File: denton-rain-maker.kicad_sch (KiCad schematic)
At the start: 73 parts, among them J1 Live(AC2), J2 Neutral(AC1), J3 SEED C3, Q1 BT136S-800E, Q2 BT136S-800E, Q3 BT136S-800E, Q4 BT136S-800E, SW1 SW_Rotary_1x8_MP, U1 MOC3063M, U2 MOC3063M, U3 MOC3063M, U4 MOC3063M, U5 LM5164DDA

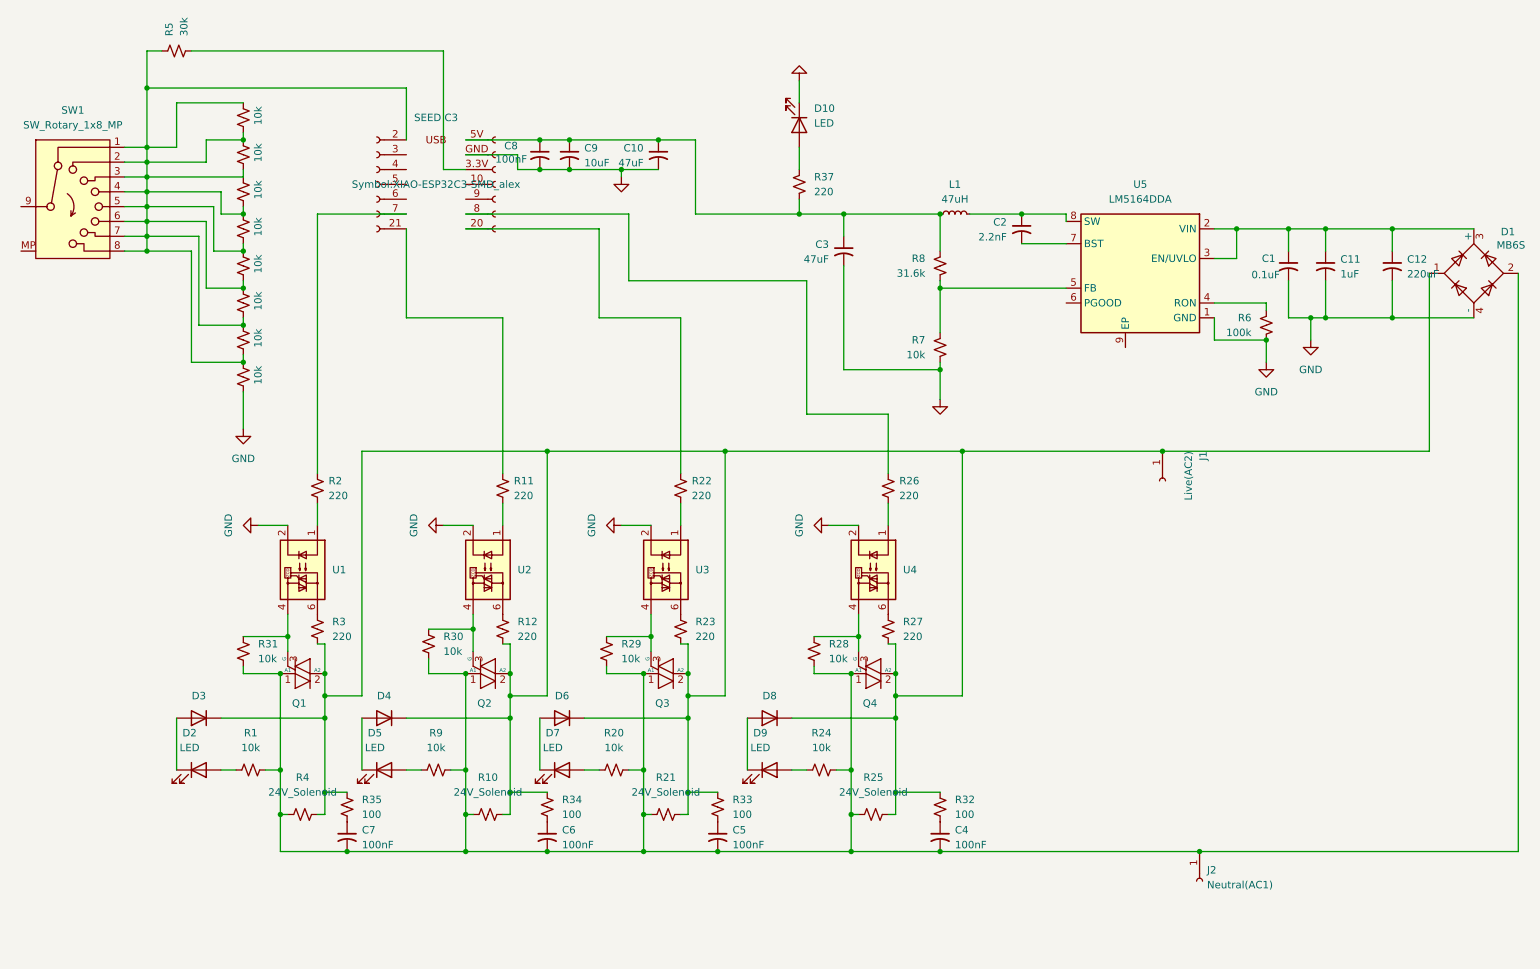
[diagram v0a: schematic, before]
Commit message: starting on layout
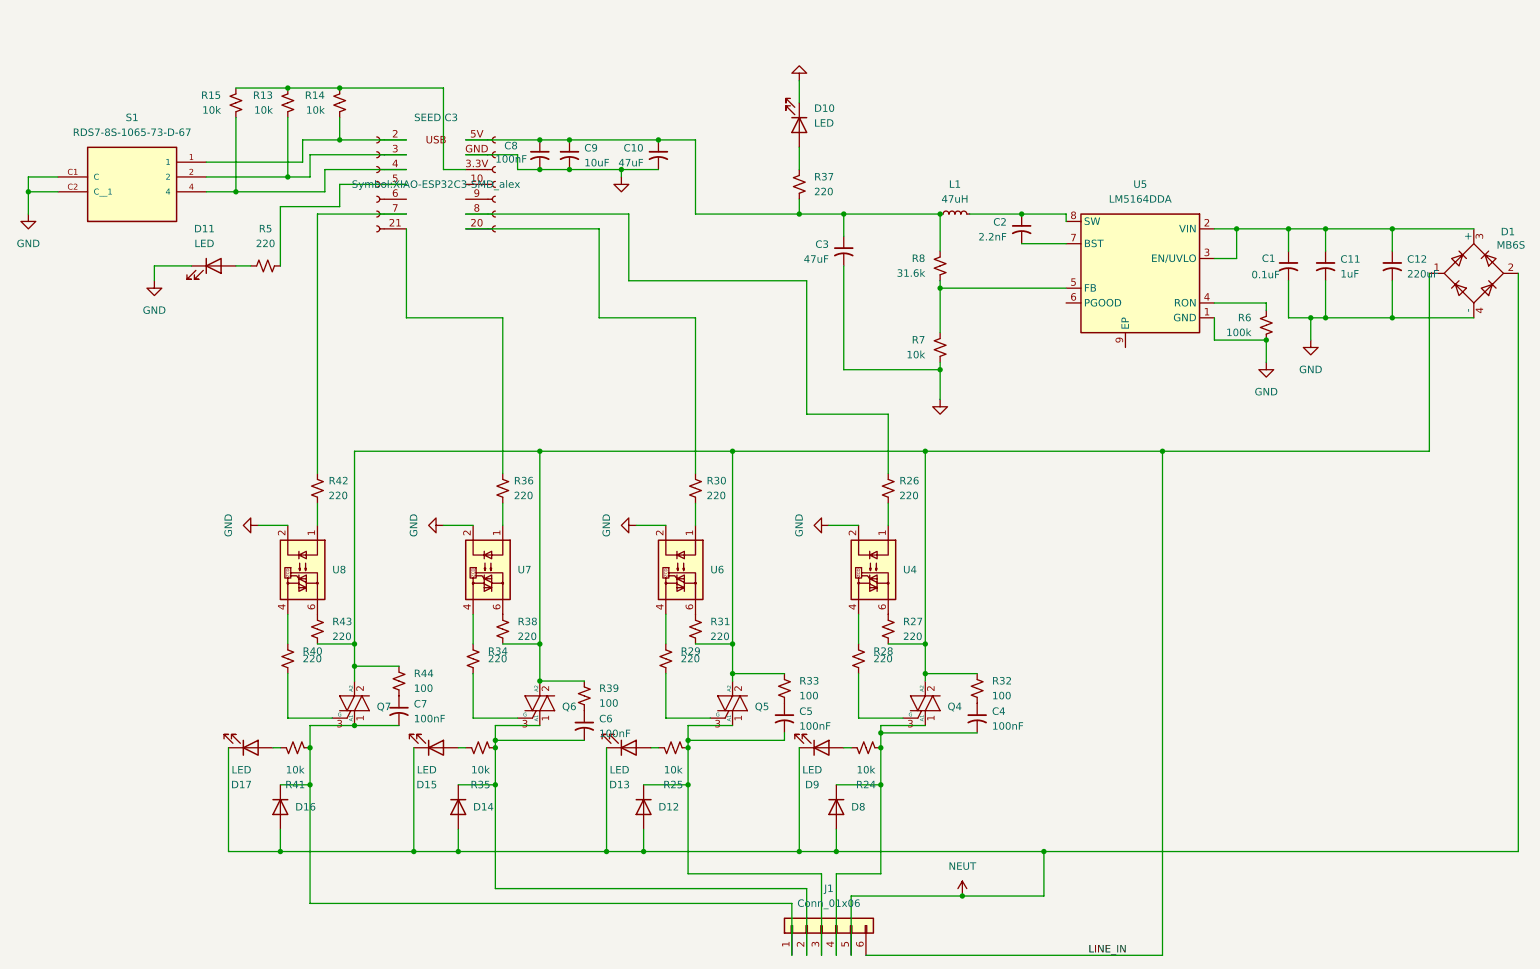
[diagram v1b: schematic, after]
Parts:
- removed D2, D5, D7: LED, LED_SMD:LED_1206_3216Metric_Pad1.42x1.75mm_HandSolder, symbol Device:LED
- removed D3, D4, D6: 1N4148W, Diode_SMD:D_SOD-123, symbol Diode:1N4148W
- removed J1: Live(AC2), Connector_PinSocket_1.27mm:PinSocket_1x01_P1.27mm_Vertical, symbol Connector:Conn_01x01_Socket
- removed J2: Neutral(AC1), Connector_PinSocket_1.27mm:PinSocket_1x01_P1.27mm_Vertical, symbol Connector:Conn_01x01_Socket
- removed Q1, Q2, Q3: BT136S-800E, Package_TO_SOT_SMD:TO-252-3_TabPin2, symbol Triac_Thyristor:BT136-800
- removed R1, R16, R17, R18, R19, R20, R9: 10k, Resistor_SMD:R_1206_3216Metric_Pad1.30x1.75mm_HandSolder, symbol Device:R_Small_US
- removed R10, R21, R4: 24V_Solenoid, symbol Device:R_Small_US
- removed R11, R12, R2, R22, R23, R3: 220, Resistor_SMD:R_1206_3216Metric_Pad1.30x1.75mm_HandSolder, symbol Device:R_Small_US
- removed SW1: SW_Rotary_1x8_MP, symbol Switch:SW_Rotary_1x8_MP
- removed U1, U2, U3: MOC3063M, Package_DIP:DIP-6_W7.62mm, symbol Relay_SolidState:MOC3063M
- added D11, D13, D15, D17: LED, LED_THT:LED_D3.0mm, symbol Device:LED
- added D12, D14, D16: 1N4148W, Diode_SMD:D_SOD-123, symbol Diode:1N4148W
- added J1: Conn_01x06, TerminalBlock_Phoenix:TerminalBlock_Phoenix_MPT-0,5-6-2.54_1x06_P2.54mm_Horizontal, symbol Connector_Generic:Conn_01x06
- added Q5, Q6, Q7: BT136S-800E, Package_TO_SOT_SMD:TO-252-3_TabPin2, symbol Triac_Thyristor:BT136-800
- added R38, R40, R42, R43: 220, Resistor_SMD:R_1206_3216Metric_Pad1.30x1.75mm_HandSolder, symbol Device:R_Small_US
- added R39, R44: 100, Resistor_SMD:R_1206_3216Metric_Pad1.30x1.75mm_HandSolder, symbol Device:R_Small_US
- added R41: 10k, Resistor_SMD:R_1206_3216Metric_Pad1.30x1.75mm_HandSolder, symbol Device:R_Small_US
- added S1: RDS7-8S-1065-73-D-67, Downloads:SW_RDS7-8S-1065-73-D-67, symbol RDS7-8S-1065-73-D-67:RDS7-8S-1065-73-D-67
- added U6, U7, U8: MOC3063M, Package_DIP:DIP-6_W7.62mm, symbol Relay_SolidState:MOC3063M
- D10: footprint (none) -> LED_THT:LED_D3.0mm
- D9: footprint LED_SMD:LED_1206_3216Metric_Pad1.42x1.75mm_HandSolder -> LED_THT:LED_D3.0mm
- R25: value 24V_Solenoid -> 10k; footprint (none) -> Resistor_SMD:R_1206_3216Metric_Pad1.30x1.75mm_HandSolder
- R28, R29, R30, R31, R36: value 10k -> 220
- R34: value 100 -> 220
- R35: value 100 -> 10k
- R5: value 30k -> 220
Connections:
- net GND: now also D11.1 (K), S1.C1 (C), S1.C2 (C__1), U6.2, U7.2, U8.2; no longer R36.1
- net at J3.20 (Pin_7): now also R30.2
- net at R31.1: now also U6.6
- net LINE_IN: now reaches D1.1, Q4.2 (A2), R27.2, R32.1, R33.1
- net LINE_IN: now also R31.2, J1.6 (Pin_6), Q5.2 (A2), Q6.2 (A2), Q7.2 (A2), R38.2, R39.1, R43.2, R44.1; no longer D8.1 (K), R25.1, R34.1, R35.1
- net at J3.7 (Pin_3): now also R42.2
- net at R28.1, U4.4: no longer Q4.3 (G)
- net NEUT: now reaches D8.2 (A), D9.1 (K)
- net NEUT: now also D1.2, D12.2 (A), D13.1 (K), D14.2 (A), D15.1 (K), D16.2 (A), D17.1 (K), J1.5 (Pin_5)
- net at R30.1: now also U6.1
- net at C6.1: now also R39.2; no longer R34.2
- net at R35.2: now also C6.2, D14.1 (K), J1.2 (Pin_2), Q6.1 (A1); no longer C7.1
- net at R29.1: now also U6.4
- net at J3.3.3V (Pin_3): now also R13.1, R14.1, R15.1; no longer R5.1
- net at J3.21 (Pin_2): now also R36.2
- net at J3.3 (Pin_7): now also R13.2, S1.2
- net at J3.4 (Pin_6): now also R15.2, S1.4
- net at J3.5 (Pin_5): now also R5.2
- new net: J3.2 (Pin_8), R14.2, S1.1
- new net: C7.1, R44.2
- new net: C7.2, D16.1 (K), J1.1 (Pin_1), Q7.1 (A1), R41.2
- new net: C5.2, D12.1 (K), J1.3 (Pin_3), Q5.1 (A1), R25.2
- new net: Q5.3 (G), R29.2
- new net: C4.2, D8.1 (K), J1.4 (Pin_4), Q4.1 (A1), R24.2
- new net: Q4.3 (G), R28.2
- new net: D17.2 (A), R41.1
- new net: R36.1, U7.1
- new net: R34.1, U7.4
- new net: R38.1, U7.6
- new net: Q6.3 (G), R34.2
- new net: D13.2 (A), R25.1
- new net: D15.2 (A), R35.1
- new net: R40.1, U8.4
- new net: Q7.3 (G), R40.2
- new net: R42.1, U8.1
- new net: R43.1, U8.6
- new net: D11.2 (A), R5.1
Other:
- moved on the sheet: C4, D8, D9, Q4, R24, R28, R32

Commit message: layout continues
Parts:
- L1: footprint (none) -> Inductor_SMD:L_Bourns_SRN6045TA
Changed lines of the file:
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@@
 			)
 		)
-		(property "Footprint" ""
+		(property "Footprint" "Inductor_SMD:L_Bourns_SRN6045TA"
 			(at 186.69 45.72 0)
 			(hide yes)
